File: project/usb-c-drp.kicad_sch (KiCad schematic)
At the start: 31 parts, among them IC6 TCPP01-M12, IC7 ECMF02-2AMX6, IC8 TCPP01-M12, Q1 STL11N3LLH6, U3 MCP73831-2-OT

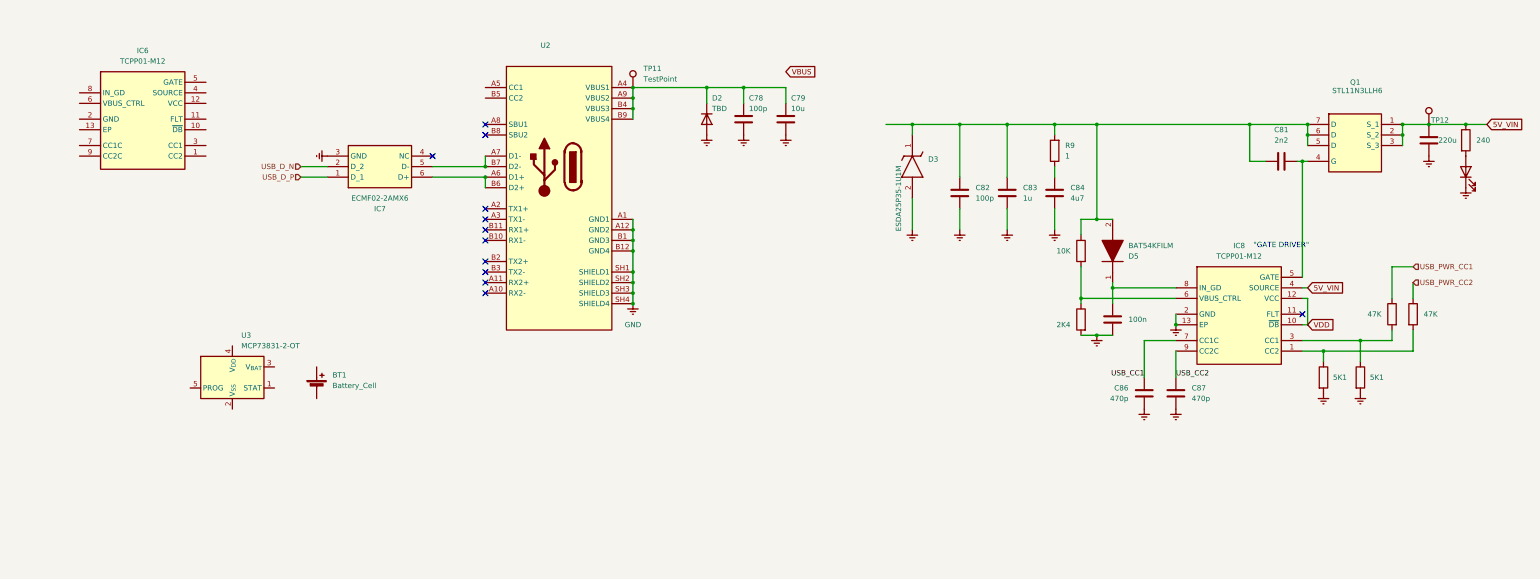
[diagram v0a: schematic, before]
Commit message: schemtic is done, need to go through BOM
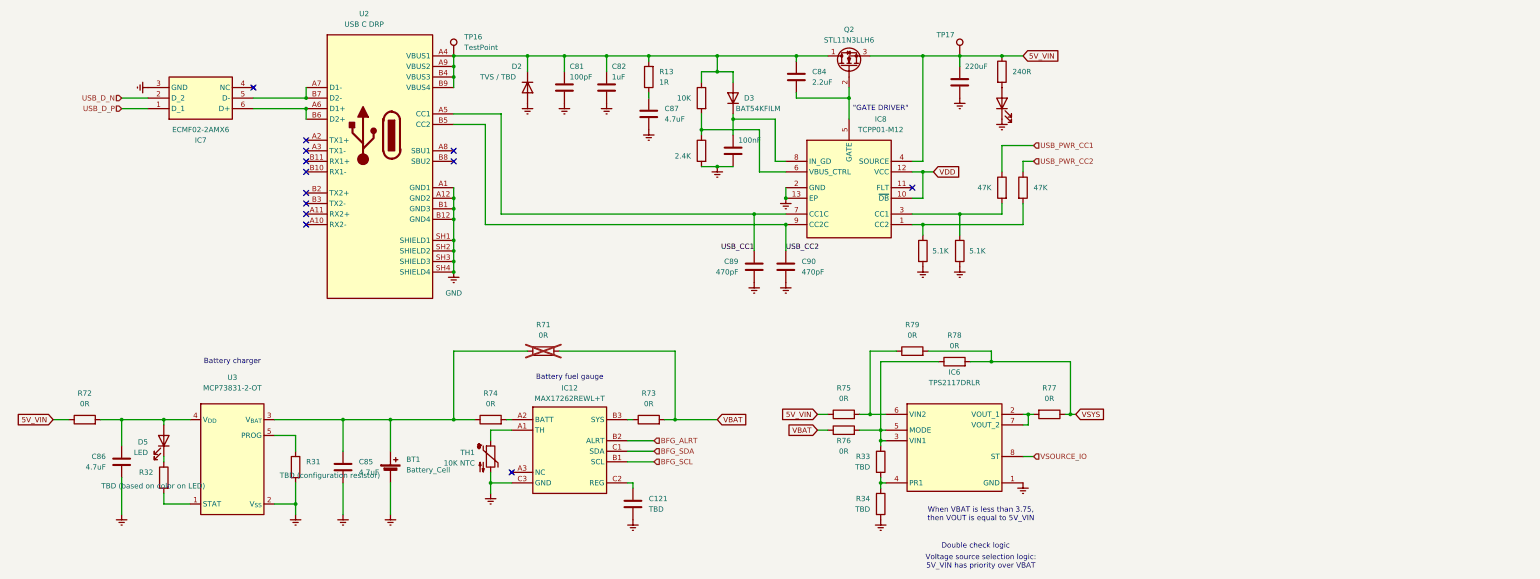
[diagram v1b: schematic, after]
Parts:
- removed C82: 100p, bozi:GRM15_T05, symbol Device:C
- removed C83: 1u, bozi:GRM15_T05, symbol Device:C
- removed D3: ESDA25P35-1U1M, ESDA25P351U1M, symbol bozi:ESDA25P35-1U1M
- removed D5: BAT54KFILM, SODFL1608X70N, symbol bozi:BAT54KFILM
- removed IC6: TCPP01-M12, QFN50P300X300X100-13N-D, symbol bozi:TCPP01-M12
- removed Q1: STL11N3LLH6, STL20N6F7, symbol bozi:STL11N3LLH6
- added C121: TBD, symbol Device:C
- added C85, C86: 4.7uF, symbol Device:C
- added D3: BAT54KFILM, bozi:SODFL1608X70N_edit, symbol Device:D
- added D5: LED, bozi:LEDC1608X70N_edit, symbol Device:LED
- added IC12: MAX17262REWL+T, BGA9C40P3X3_147X145X69, symbol bozi:MAX17262REWL+T
- added IC6: TPS2117DRLR, SOTFL50P160X60-8N, symbol bozi:TPS2117DRLR
- added Q2: STL11N3LLH6, bozi:STL20N6F7_edit, symbol Transistor_FET:Q_NMOS_DGS
- added R31: TBD (configuration resistor), symbol Device:R
- added R32: TBD (based on color on LED), symbol Device:R
- added R33, R34: TBD, symbol Device:R
- added R71, R72, R73, R74, R75, R76, R77, R78, R79: 0R, bozi:RESC1005X37N_edit, symbol Device:R
- added TH1: 10K NTC, bozi:THRMC1005X55N, symbol Device:Thermistor_NTC
- BT1: Manufacturer_Name (none) -> x; Manufacturer_Part_Number (none) -> x
- C81: renamed from C78; value 100p -> 100pF; Manufacturer_Name (none) -> Murata Electronics; Manufacturer_Part_Number (none) -> GRM0335C1H101JA01D
- C82: renamed from C79; value 10u -> 1uF; footprint (none) -> bozi:GRM15_T05; Manufacturer_Name (none) -> Murata Electronics; Manufacturer_Part_Number (none) -> GRM155R61E105KA12D
- C83: renamed from C80; value 220u -> 220uF; Manufacturer_Name (none) -> Murata Electronics
- C84: renamed from C81; value 2n2 -> 2.2uF; Manufacturer_Name (none) -> Murata Electronics
- C87: renamed from C84; value 4u7 -> 4.7uF; Manufacturer_Name (none) -> Murata Electronics
- C88: renamed from C85; value 100n -> 100nF; Manufacturer_Name (none) -> Murata Electronics
- C89: renamed from C86; value 470p -> 470pF; Manufacturer_Name (none) -> Murata Electronics
- C90: renamed from C87; value 470p -> 470pF; Manufacturer_Name (none) -> Murata Electronics
- D2: value TBD -> TVS / TBD
- D4: Manufacturer_Name (none) -> Würth Elektronik
- R12: renamed from R8; value 240 -> 240R; Manufacturer_Name (none) -> YAGEO
- R13: renamed from R9; value 1 -> 1R; Manufacturer_Name (none) -> Yageo
- R14: renamed from R10; Manufacturer_Name (none) -> YAGEO
- R15: renamed from R11; Manufacturer_Name (none) -> YAGEO
- R16: renamed from R12; Manufacturer_Name (none) -> YAGEO
- R17: renamed from R13; value 2K4 -> 2.4K; Manufacturer_Name (none) -> YAGEO
- R18: renamed from R14; value 5K1 -> 5.1K; Manufacturer_Name (none) -> YAGEO
- R19: renamed from R15; value 5K1 -> 5.1K; Manufacturer_Name (none) -> YAGEO
- U2: value ~ -> USB C DRP; footprint (none) -> bozi:2012670005_edit; Manufacturer_Name (none) -> Molex; Manufacturer_Part_Number (none) -> 2012670005
- U3: symbol Battery_Management:MCP73831-2-OT -> bozi:MCP73831-2-OT; Manufacturer_Name (none) -> Microchip Technology; Manufacturer_Part_Number (none) -> MCP73831-2ATI/MC-ND
- renumbered TP11 to TP16, TP12 to TP17
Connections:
- net 5V_VIN: now also Q2.3 (S), R72.1, R75.1
- net GND: now also BT1.2 (-), U3.2 (V_{SS}), C121.2, C85.2, C86.2, IC12.C3 (GND), R31.2, TH1.2
- net GNDREF: now also IC6.1 (GND), R34.2
- net USB_CC1: now also U2.A5 (CC1)
- net USB_CC2: now also U2.B5 (CC2)
- net at C81.1, C82.1, D2.1 (K)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: now also C84.2, R13.2, R14.1, D3.2 (A), Q2.1 (D)
- net at IC8.5 (GATE): now also C84.1, Q2.2 (G); no longer C84.2
- net at C88.2, IC8.8 (IN_GD): now also D3.1 (K)
- net at BT1.1 (+): now also U3.3 (V_{BAT}), C85.1, R71.1, R74.1
- net at U3.1 (STAT): now also R32.2
- net at U3.4 (V_{DD}): now also C86.1, D5.2 (A), R72.2
- net at U3.5 (PROG): now also R31.1
- new net: IC6.3 (VIN1), IC6.5 (MODE), R33.1, R76.2, R78.1
- new net: IC12.B3 (SYS), R73.1
- new net: IC6.4 (PR1), R33.2, R34.1
- new net: C121.1, IC12.C2 (REG)
- new net: IC6.2 (VOUT_1), IC6.7 (VOUT_2), R77.2
- new net: IC6.6 (VIN2), R75.2, R79.1
- new net: D5.1 (K), R32.1
- new net: IC12.A2 (BATT), R74.2
- new net: IC12.A1 (TH), TH1.1
- new net BFG_ALRT: IC12.B2 (ALRT)
- new net BFG_SCL: IC12.B1 (SCL)
- new net BFG_SDA: IC12.C1 (SDA)
- new net VBAT: R71.2, R73.2, R76.1
- new net VSOURCE_IO: IC6.8 (ST)
- new net VSYS: R77.1, R78.2, R79.2
- no-connect marks 12 -> 13
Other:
- note added: "Battery charger"
- note added: "Battery fuel gauge"
- note added: "Double check logic"
- note added: "Voltage source selection logic: 5V_VIN has priority over VBAT"
- note added: "When VBAT is less than 3.75, then VOUT is equal to 5V_VIN"
- moved on the sheet: BT1, C81, C82, C84, C87, C89, C90, D2, IC7, IC8, R13, TP16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
